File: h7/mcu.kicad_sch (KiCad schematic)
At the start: 1 part, among them U201 STM32H743VITx

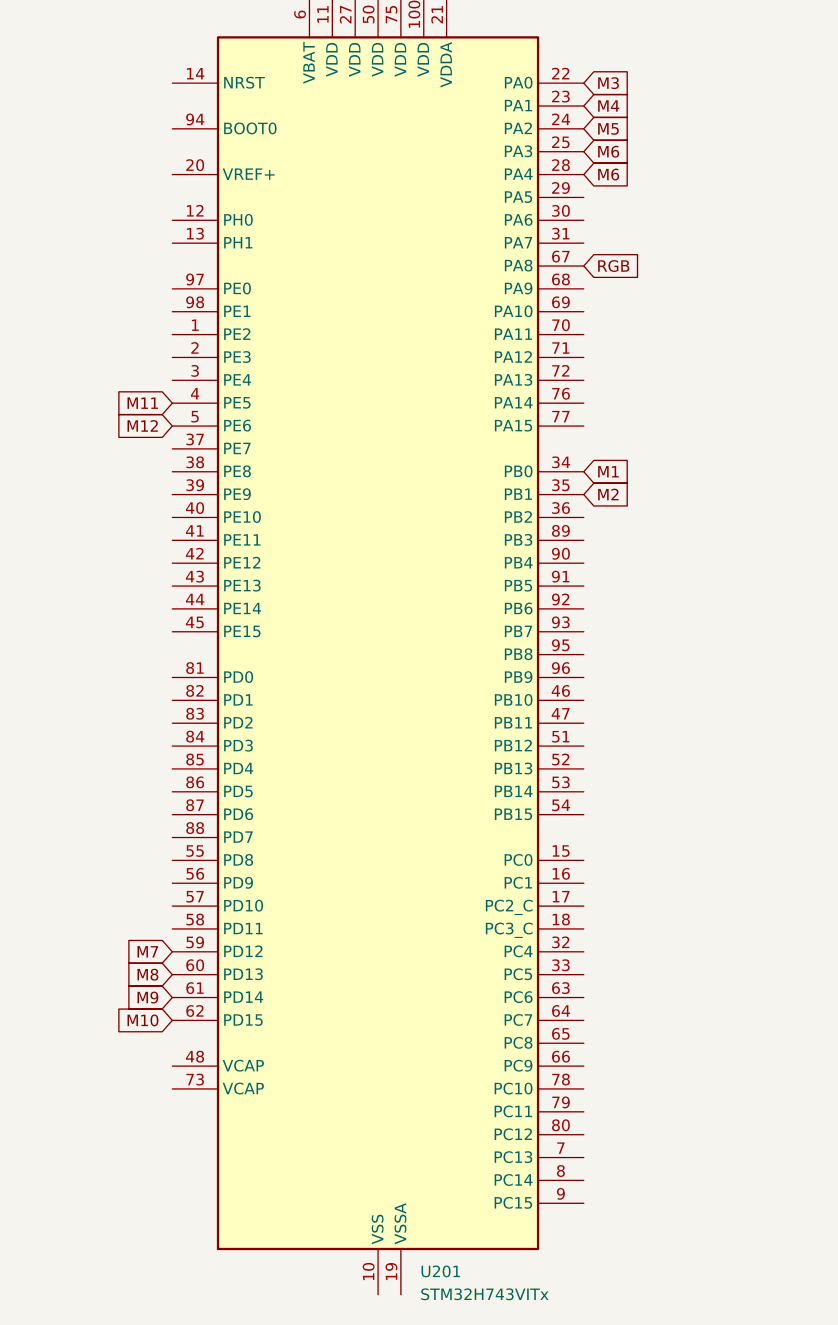
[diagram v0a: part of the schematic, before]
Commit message: todays progress with schematic and pinout
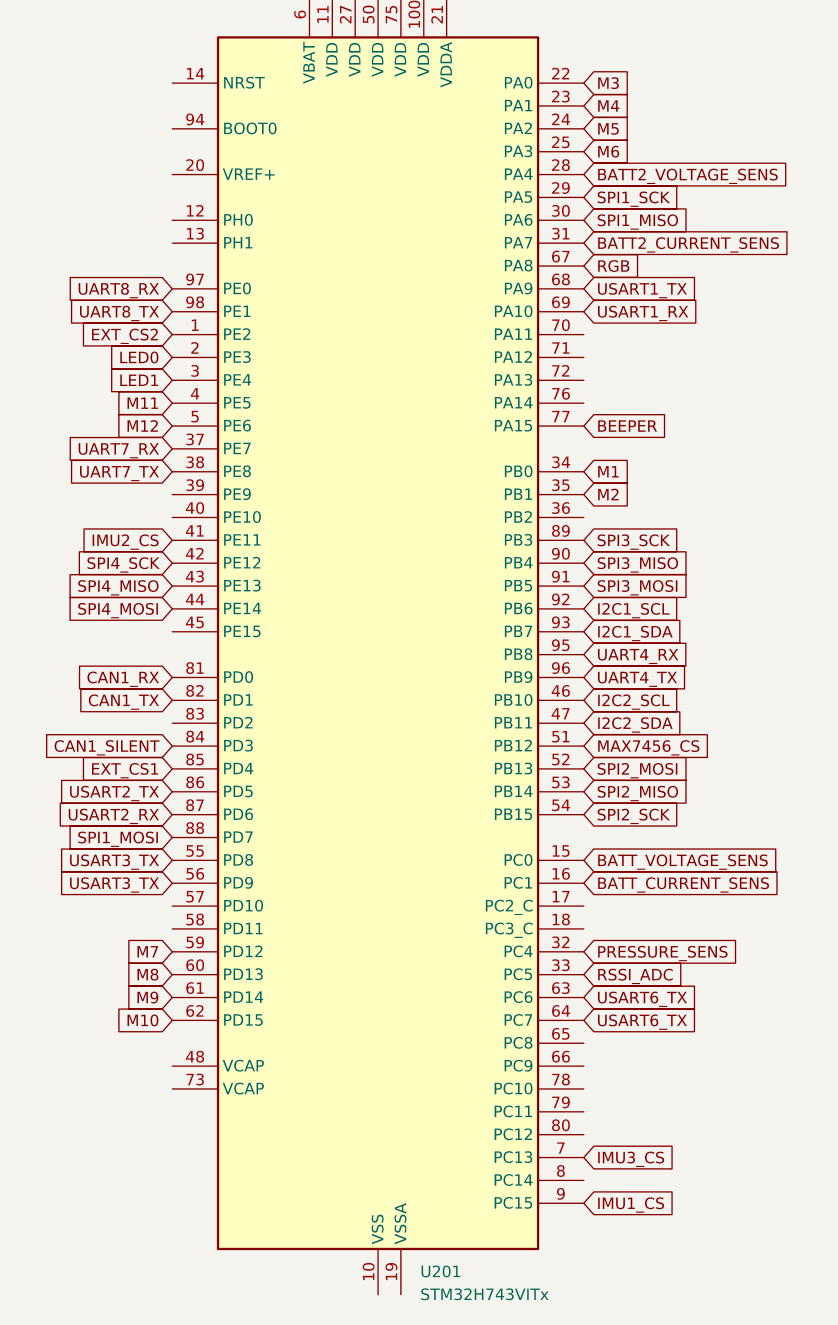
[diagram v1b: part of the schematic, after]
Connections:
- net M6: no longer U201.28 (PA4)
- net EXT_CS2: now reaches U201.1 (PE2)
- net BATT_VOLTAGE_SENS: now reaches U201.15 (PC0)
- net BATT_CURRENT_SENS: now reaches U201.16 (PC1)
- net LED0: now reaches U201.2 (PE3)
- net SPI1_SCK: now reaches U201.29 (PA5)
- net LED1: now reaches U201.3 (PE4)
- net SPI1_MISO: now reaches U201.30 (PA6)
- net BATT2_CURRENT_SENS: now reaches U201.31 (PA7)
- net PRESSURE_SENS: now reaches U201.32 (PC4)
- net RSSI_ADC: now reaches U201.33 (PC5)
- net UART7_RX: now reaches U201.37 (PE7)
- net UART7_TX: now reaches U201.38 (PE8)
- net IMU2_CS: now reaches U201.41 (PE11)
- net SPI4_SCK: now reaches U201.42 (PE12)
- net SPI4_MISO: now reaches U201.43 (PE13)
- net SPI4_MOSI: now reaches U201.44 (PE14)
- net I2C2_SCL: now reaches U201.46 (PB10)
- net I2C2_SDA: now reaches U201.47 (PB11)
- net MAX7456_CS: now reaches U201.51 (PB12)
- net SPI2_MOSI: now reaches U201.52 (PB13)
- net SPI2_MISO: now reaches U201.53 (PB14)
- net SPI2_SCK: now reaches U201.54 (PB15)
- net USART3_TX: now reaches U201.55 (PD8)
- net USART3_TX: now also U201.56 (PD9)
- net USART6_TX: now reaches U201.63 (PC6)
- net USART6_TX: now also U201.64 (PC7)
- net USART1_TX: now reaches U201.68 (PA9)
- net USART1_RX: now reaches U201.69 (PA10)
- net IMU3_CS: now reaches U201.7 (PC13)
- net BEEPER: now reaches U201.77 (PA15)
- net CAN1_RX: now reaches U201.81 (PD0)
- net CAN1_TX: now reaches U201.82 (PD1)
- net CAN1_SILENT: now reaches U201.84 (PD3)
- net EXT_CS1: now reaches U201.85 (PD4)
- net USART2_TX: now reaches U201.86 (PD5)
- net USART2_RX: now reaches U201.87 (PD6)
- net SPI1_MOSI: now reaches U201.88 (PD7)
- net SPI3_SCK: now reaches U201.89 (PB3)
- net IMU1_CS: now reaches U201.9 (PC15)
- net SPI3_MISO: now reaches U201.90 (PB4)
- net SPI3_MOSI: now reaches U201.91 (PB5)
- net I2C1_SCL: now reaches U201.92 (PB6)
- net I2C1_SDA: now reaches U201.93 (PB7)
- net UART4_RX: now reaches U201.95 (PB8)
- net UART4_TX: now reaches U201.96 (PB9)
- net UART8_RX: now reaches U201.97 (PE0)
- net UART8_TX: now reaches U201.98 (PE1)
- new net BATT2_VOLTAGE_SENS: U201.28 (PA4)

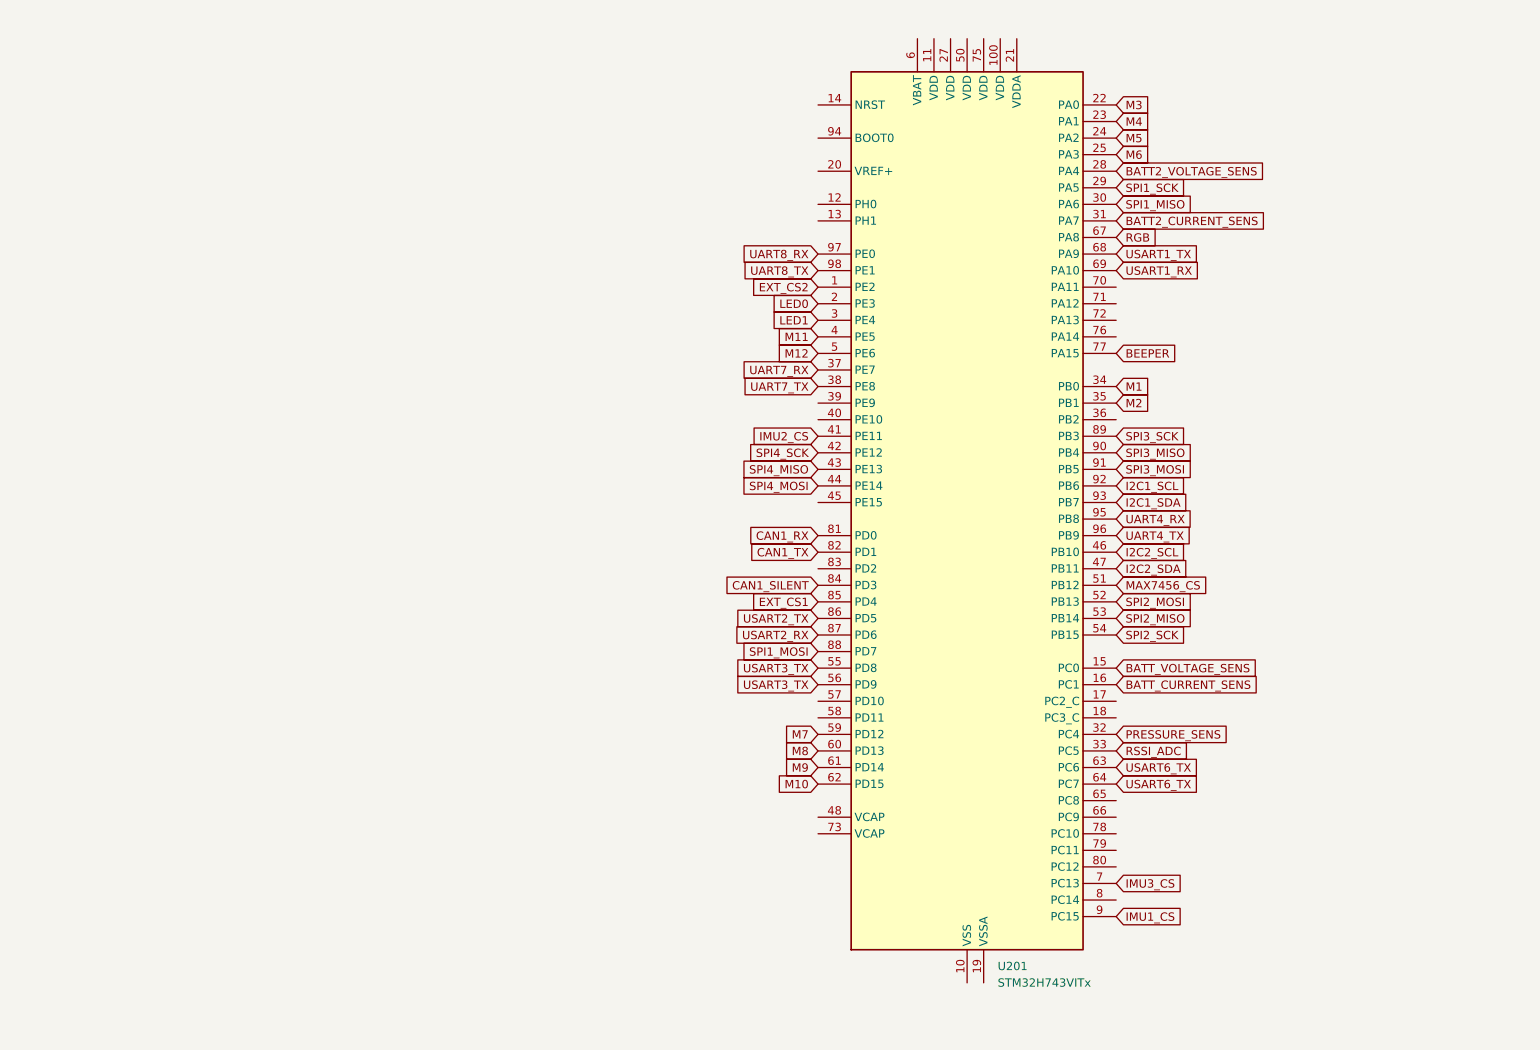
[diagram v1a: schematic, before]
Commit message: todays progresss
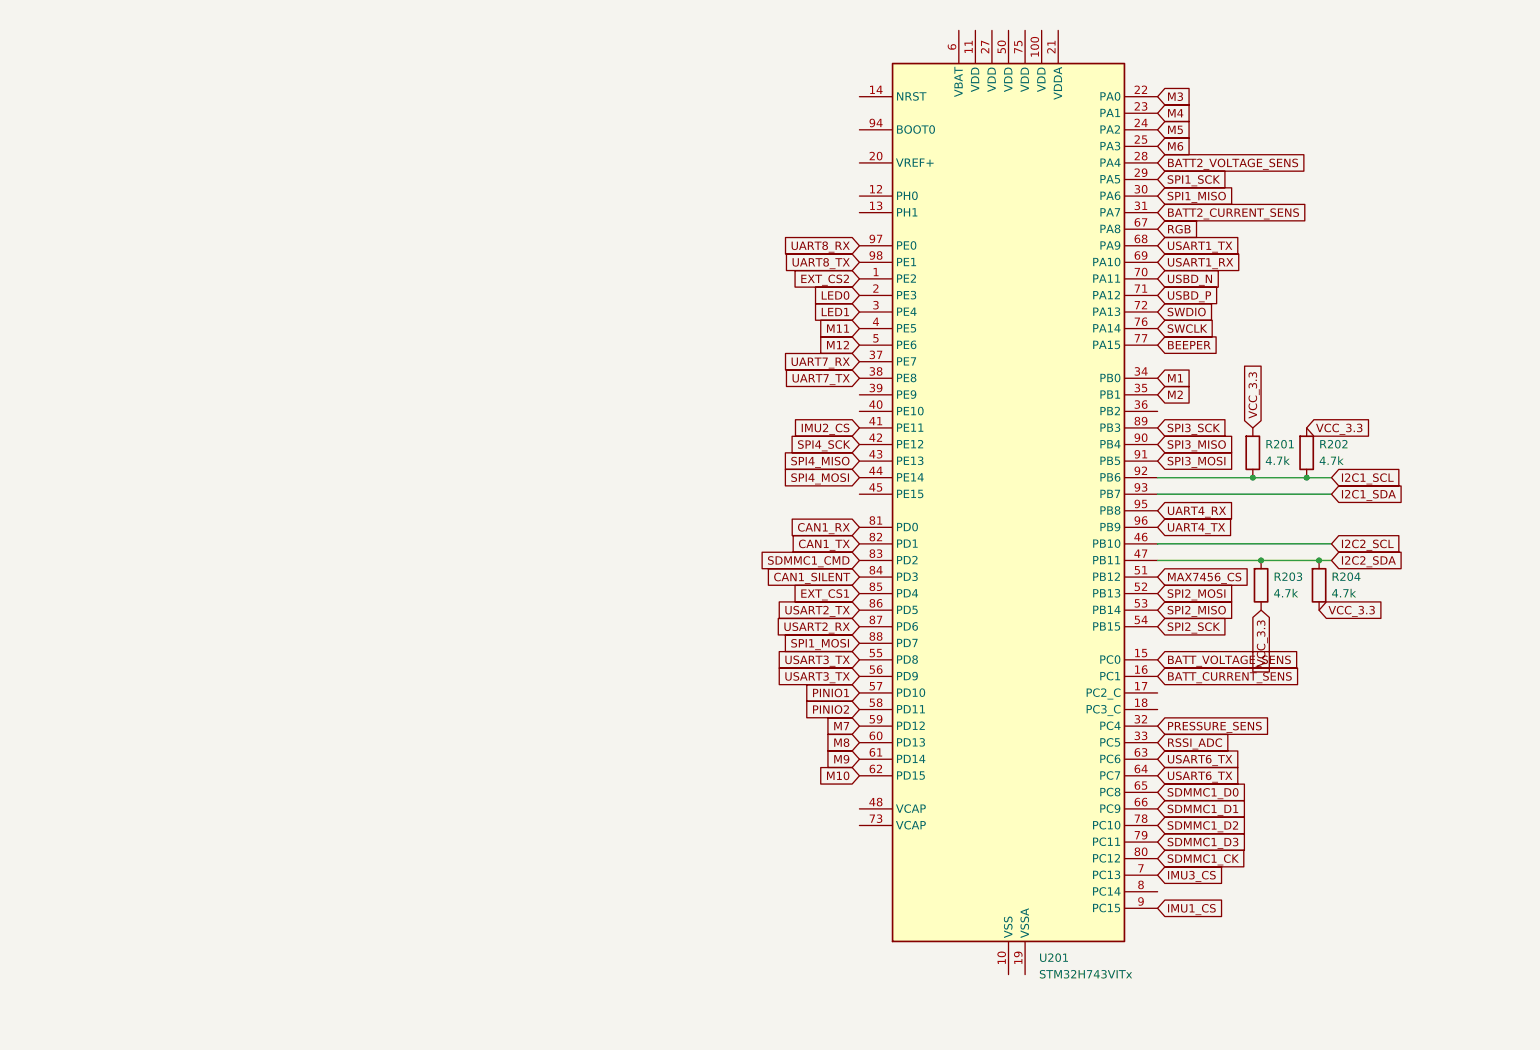
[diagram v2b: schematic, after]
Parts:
- added R201, R202, R203, R204: 4.7k, PCM_Resistor_SMD_AKL:R_0402_1005Metric, symbol PCM_Resistor_AKL:R_0402
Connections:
- net I2C1_SCL: now also R201.2, R202.2
- net I2C2_SDA: now also R203.1, R204.1
- net PINIO1: now reaches U201.57 (PD10)
- net PINIO2: now reaches U201.58 (PD11)
- net SDMMC1_D0: now reaches U201.65 (PC8)
- net SDMMC1_D1: now reaches U201.66 (PC9)
- net USBD_N: now reaches U201.70 (PA11)
- net USBD_P: now reaches U201.71 (PA12)
- net SWDIO: now reaches U201.72 (PA13)
- net SWCLK: now reaches U201.76 (PA14)
- net SDMMC1_D2: now reaches U201.78 (PC10)
- net SDMMC1_D3: now reaches U201.79 (PC11)
- net SDMMC1_CK: now reaches U201.80 (PC12)
- net SDMMC1_CMD: now reaches U201.83 (PD2)
- new net VCC_3.3: R201.1, R202.1, R203.2, R204.2
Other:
- moved on the sheet: U201

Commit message: before final
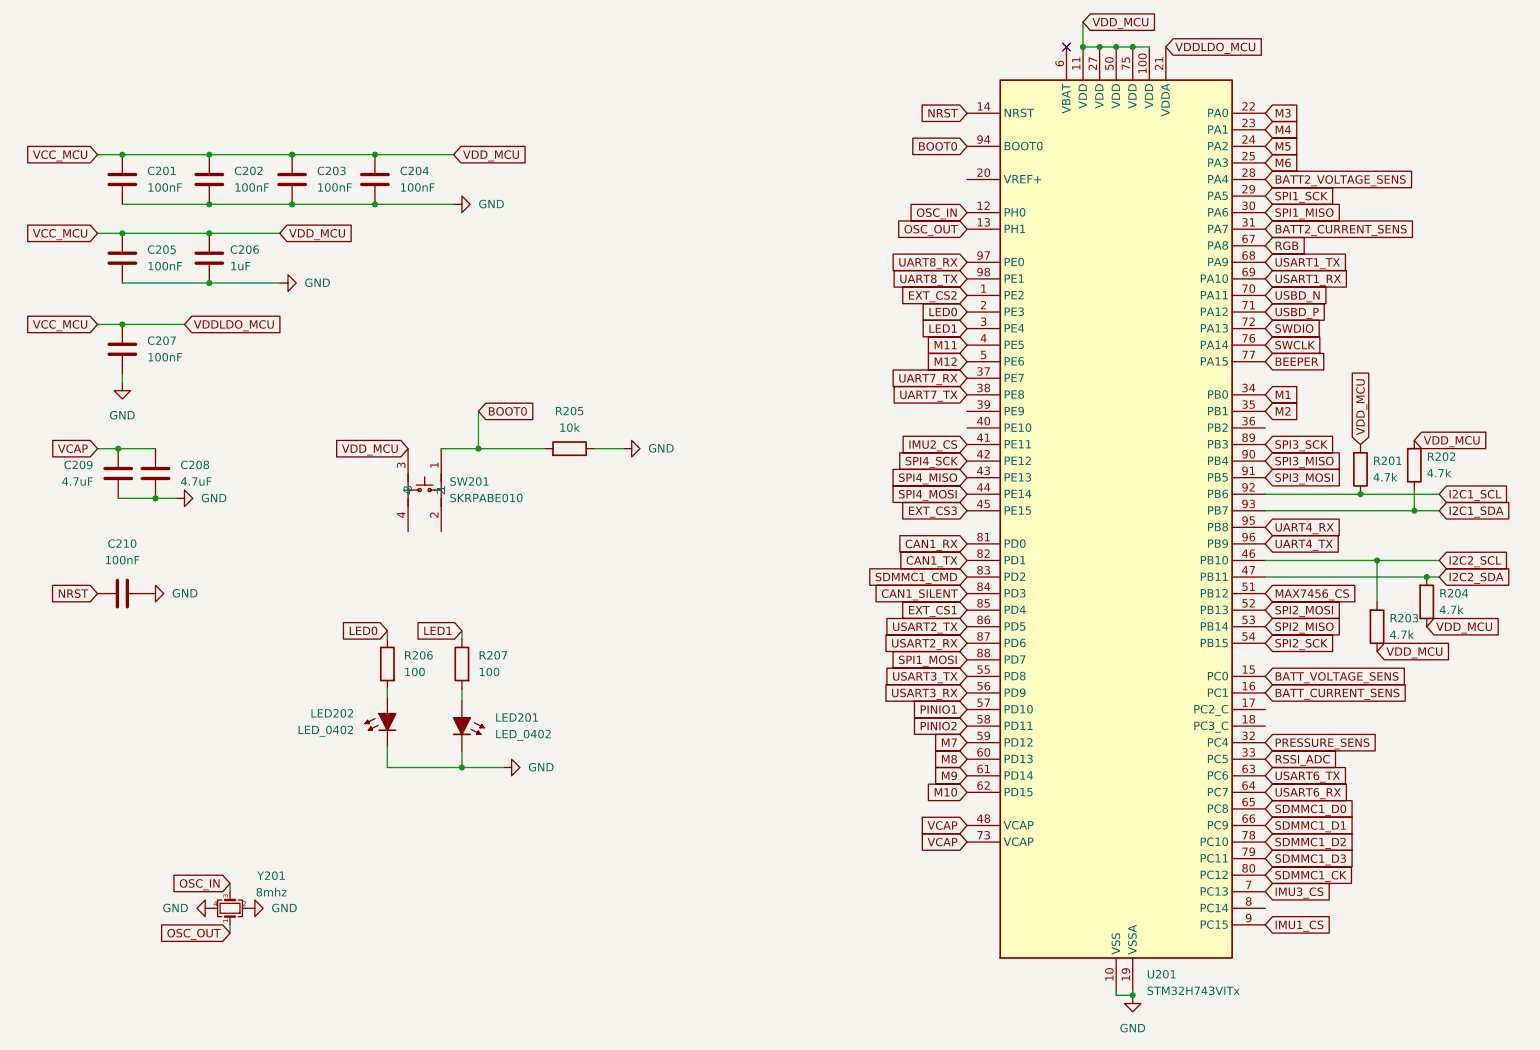
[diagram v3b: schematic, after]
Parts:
- added C201, C202, C203, C204, C205, C207, C210: 100nF, PCM_Capacitor_SMD_AKL:C_0402_1005Metric, symbol PCM_Capacitor_AKL:C_0402
- added C206: 1uF, PCM_Capacitor_SMD_AKL:C_0402_1005Metric, symbol PCM_Capacitor_AKL:C_0402
- added C208, C209: 4.7uF, PCM_Capacitor_SMD_AKL:C_0402_1005Metric, symbol PCM_Capacitor_AKL:C_0402
- added LED201, LED202: LED_0402, PCM_LED_SMD_AKL:LED_0402_1005Metric, symbol PCM_LED_AKL:LED_0402
- added R205: 10k, PCM_Resistor_SMD_AKL:R_0402_1005Metric, symbol PCM_Resistor_AKL:R_0402
- added R206, R207: 100, PCM_Resistor_SMD_AKL:R_0402_1005Metric, symbol PCM_Resistor_AKL:R_0402
- added SW201: SKRPABE010, easyeda2kicad:KEY-SMD_4P-L4.2-W3.2-P2.20-LS4.6, symbol easyeda2kicad:SKRPABE010
- added Y201: 8mhz, Crystal:Crystal_SMD_2520-4Pin_2.5x2.0mm, symbol Device:Crystal_GND24_Small
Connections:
- net VCC_3.3 is gone; now on net VCC_MCU: R201.1, R202.1, R203.2, R204.2
- net I2C1_SCL: no longer R202.2
- net I2C1_SDA: now also R202.2
- net I2C2_SCL: now also R203.1
- net I2C2_SDA: no longer R203.1
- net LED0: now also R206.2
- net LED1: now also R207.2
- net USART3_TX: no longer U201.56 (PD9)
- net USART6_TX: no longer U201.64 (PC7)
- net GND: now reaches U201.10 (VSS), U201.26 (VSS), U201.49 (VSS), U201.74 (VSS), U201.99 (VSS)
- net GND: now also U201.19 (VSSA), C201.2, C202.2, C203.2, C204.2, C205.2, C206.2, C207.2, C208.2, C209.2, C210.2, LED201.1 (K), LED202.1 (K), R205.2, Y201.2, Y201.4
- net VCC_MCU: now reaches U201.100 (VDD)
- net VCC_MCU: now also U201.11 (VDD), U201.21 (VDDA), U201.27 (VDD), U201.50 (VDD), U201.75 (VDD), C201.1, C202.1, C203.1, C204.1, C205.1, C206.1, C207.1, SW201.3
- net OSC_IN: now reaches U201.12 (PH0)
- net OSC_IN: now also Y201.3
- net OSC_OUT: now reaches U201.13 (PH1)
- net OSC_OUT: now also Y201.1
- net NRST: now reaches U201.14 (NRST)
- net NRST: now also C210.1
- net EXT_CS3: now reaches U201.45 (PE15)
- net VCAP: now reaches U201.48 (VCAP)
- net VCAP: now also U201.73 (VCAP), C208.1, C209.1
- net BOOT0: now reaches U201.94 (BOOT0)
- net BOOT0: now also R205.1, SW201.1
- new net: LED202.2 (A), R206.1
- new net: LED201.2 (A), R207.1
- new net USART3_RX: U201.56 (PD9)
- new net USART6_RX: U201.64 (PC7)
- no-connect marks 0 -> 1
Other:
- moved on the sheet: R201, R202, R203, R204, U201
